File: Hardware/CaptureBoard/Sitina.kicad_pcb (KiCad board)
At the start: 2 copper layers, 64 x 38 mm, 211 parts, among them J100 Conn_01x30_MountingPin, Q1000 DMC3071LVT, Q1001 DMC3071LVT, Q1002 DMC3071LVT, Q1003 DMC3071LVT, Q1100 BC847BPN, U1 ADA4800, U10 LT1964-BYP, U11 LT1964-BYP, U1200 KAI-1100x, U2 ADA4800, U4 LT3472, U5 LT3472, U6 LT3472, U7 LT3023, U8 LT3023, U800 AD9990, U900 74LCX541BQX, U901 74LCX541BQX, U902 74LCX541BQX, U903 74LCX541BQX, Y800 30MHz

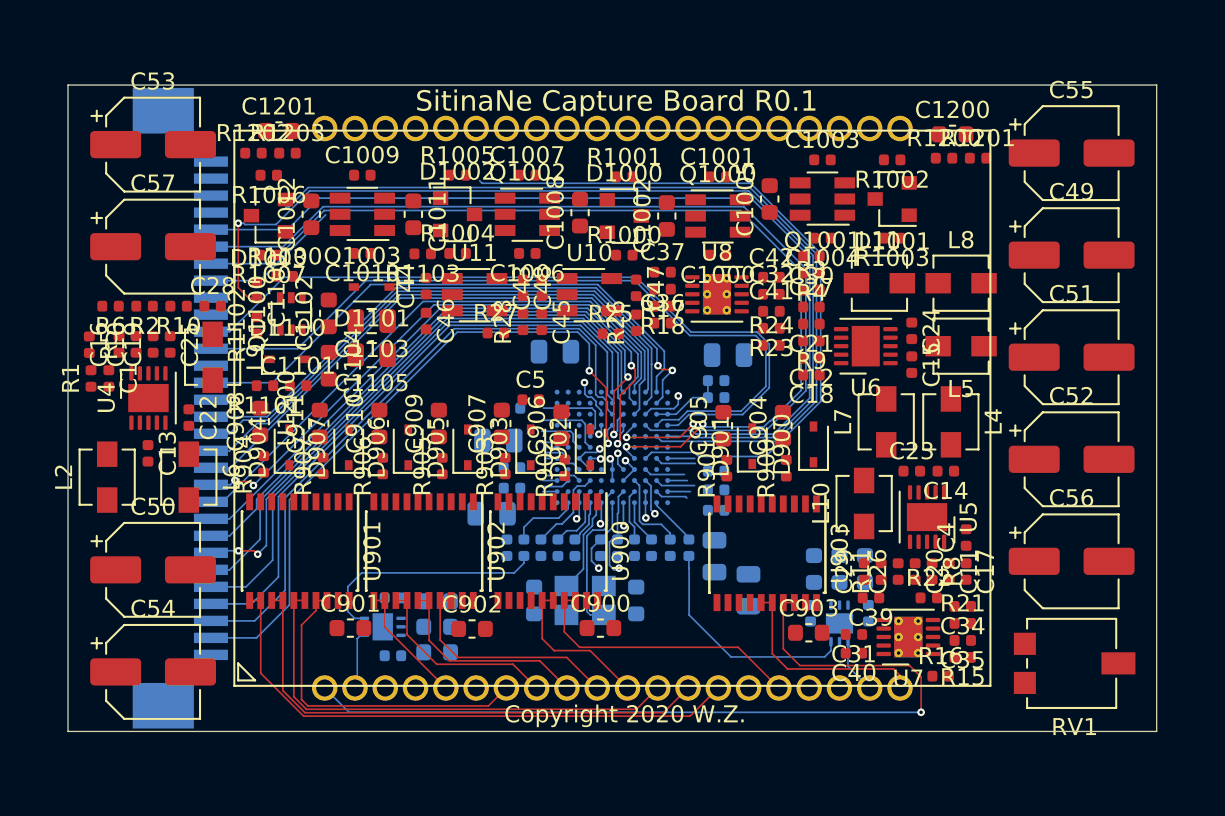
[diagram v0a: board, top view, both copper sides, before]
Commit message: pcb: wip
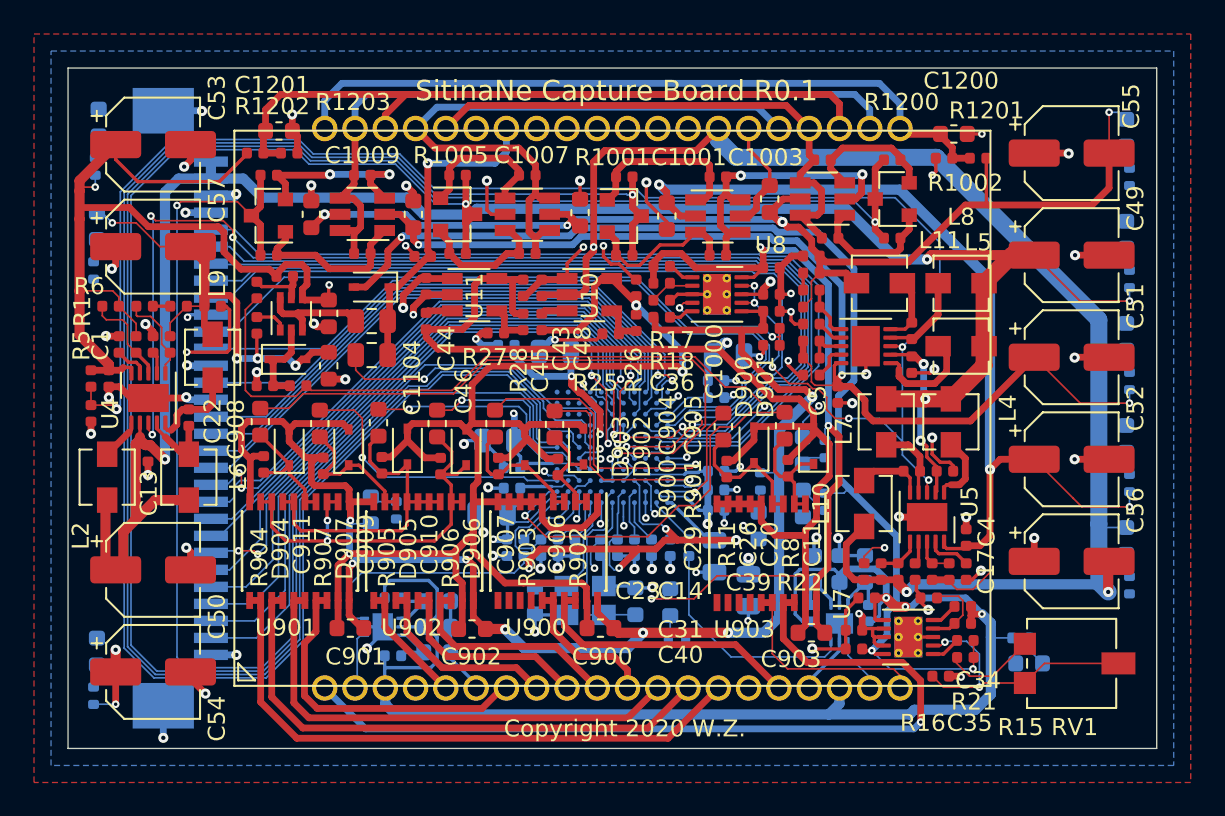
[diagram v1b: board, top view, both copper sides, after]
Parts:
- added D1: LED, Diode_SMD:D_0603_1608Metric, B.Cu at (175.2, 90.8)
- added D10: LED, Diode_SMD:D_0603_1608Metric, B.Cu at (156.2, 106.6)
- added D11: LED, Diode_SMD:D_0603_1608Metric, B.Cu at (153.6, 107.9)
- added D12: LED, Diode_SMD:D_0603_1608Metric, B.Cu at (156.2, 103.5)
- added D13: LED, Diode_SMD:D_0603_1608Metric, B.Cu at (130.8, 107.0)
- added D14: LED, Diode_SMD:D_0603_1608Metric, B.Cu at (148.4, 112.4)
- added D2: LED, Diode_SMD:D_0603_1608Metric, B.Cu at (175.2, 96.8)
- added D3: LED, Diode_SMD:D_0603_1608Metric, B.Cu at (175.2, 102.8)
- added D4: LED, Diode_SMD:D_0603_1608Metric, B.Cu at (114.8, 84.2)
- added D5: LED, Diode_SMD:D_0603_1608Metric, B.Cu at (114.7, 115.3)
- added D6: LED, Diode_SMD:D_0603_1608Metric, B.Cu at (175.2, 84.8)
- added D7: LED, Diode_SMD:D_0603_1608Metric, B.Cu at (175.2, 108.8)
- added D8: LED, Diode_SMD:D_0603_1608Metric, B.Cu at (114.7, 90.3)
- added D9: LED, Diode_SMD:D_0603_1608Metric, B.Cu at (169.5, 116.0)
- added R12: 3.3K, Resistor_SMD:R_0402_1005Metric, B.Cu at (175.4, 99.4)
- added R13: 4.7K, Resistor_SMD:R_0402_1005Metric, B.Cu at (175.4, 105.4)
- added R14: 10K, Resistor_SMD:R_0402_1005Metric, B.Cu at (114.6, 86.8)
- added R19: 2K, Resistor_SMD:R_0402_1005Metric, B.Cu at (114.5, 117.9)
- added R20: 4.7K, Resistor_SMD:R_0402_1005Metric, B.Cu at (175.4, 87.4)
- added R29: 4.7K, Resistor_SMD:R_0402_1005Metric, B.Cu at (175.4, 111.4)
- added R30: 7.5K, Resistor_SMD:R_0402_1005Metric, B.Cu at (114.5, 92.9)
- added R31: 3.3K, Resistor_SMD:R_0402_1005Metric, B.Cu at (169.0, 114.5)
- added R32: 4.7K, Resistor_SMD:R_0402_1005Metric, B.Cu at (157.5, 106.5)
- added R33: 10K, Resistor_SMD:R_0402_1005Metric, B.Cu at (153.7, 105.3)
- added R34: 2K, Resistor_SMD:R_0402_1005Metric, B.Cu at (157.5, 103.4)
- added R35: 3.3K, Resistor_SMD:R_0402_1005Metric, B.Cu at (132.3, 107.0)
- added R36: 2K, Resistor_SMD:R_0402_1005Metric, B.Cu at (148.8, 114.5)
- added R7: 3.3K, Resistor_SMD:R_0402_1005Metric, B.Cu at (175.4, 93.4)
- R1201: value 20K/1% -> 51K/1%
- R1202: value 60.4K/1% -> 100K/1%
- R1203: value 200K/1% -> 154K/1%
- moved C5 18.1 mm to (158.2, 100.2), turned to 270 degrees
- moved C831 5.95 mm to (146.3, 112.3), turned to 270 degrees
- moved C832 5.95 mm to (140.4, 112.3), turned to 90 degrees
- moved R5 4.04 mm to (114.3, 101.3), turned to 90 degrees
- moved C817 3.72 mm to (138.8, 97.3)
- moved C905 3.60 mm to (155.1, 102.0)
- moved D901 3.60 mm to (156.8, 103.2)
- moved R901 3.60 mm to (155.3, 104.5)
- moved C909 3.55 mm to (131.2, 101.8)
- moved D905 3.55 mm to (132.9, 103.2)
- moved R905 3.55 mm to (131.4, 104.3)
- moved C904 3.50 mm to (151.5, 102.1)
- moved D900 3.50 mm to (153.3, 103.2)
- moved R900 3.50 mm to (151.7, 104.6)
- moved D906 3.40 mm to (136.4, 103.3)
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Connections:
- C1200 pad 1: /ccd/VOD -> GND
- C1200 pad 2: -4V -> /ccd/VOD
- J100 pad 23: /afe/AFE_SDATA -> /afe/AFE_SCK
- J100 pad 24: /afe/AFE_SCK -> /afe/AFE_RST
- J100 pad 25: /afe/AFE_RST -> /afe/AFE_SYNC
- J100 pad 26: /afe/AFE_SYNC -> /afe/AFE_SDATA
- R1201 pad 2: -4V -> -9V
- R1202 pad 1: +15V -> +19V
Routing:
- net GND: track 20.5 -> 185.7 mm, vias 10 -> 88
- net +SYS: track 0.00 -> 123.2 mm, vias 0 -> 6
- net -4V: track 0.00 -> 122.3 mm, vias 0 -> 4
- net /afe/AFE_V2: track 1.74 -> 120.2 mm, vias 0 -> 1
- net +19V: track 0.00 -> 105.8 mm, vias 0 -> 3
- net /afe/AFE_V2_3rd: track 0.70 -> 104.6 mm, vias 0 -> 1
- net Net-(R1-Pad1): track 0.00 -> 101.4 mm, vias 0 -> 7
- net -8V: track 0.00 -> 100.9 mm, vias 0 -> 4
- net /afe/AFE_V1: track 2.85 -> 97.6 mm, vias 0 -> 1
- net +15V: track 0.00 -> 89.0 mm, vias 0 -> 3
- net -3V5: track 0.00 -> 76.3 mm, vias 0 -> 1
- net -9V: track 0.00 -> 71.6 mm, vias 0 -> 4
- net /afe/AFE_FDG: track 4.72 -> 76.3 mm, vias 0 -> 1
- net +2V: track 0.00 -> 68.8 mm, vias 0 -> 6
- net VAB: track 0.00 -> 68.2 mm, vias 0 -> 3
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- added copper zone on In1.Cu, net +3V3
- added copper zone on B.Cu, net GND
- added copper zone on F.Cu, net GND
- added copper zone on In2.Cu, net GND
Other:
- board size 64 x 38 mm -> 64 x 40 mm
- copper layers 2 -> 4
